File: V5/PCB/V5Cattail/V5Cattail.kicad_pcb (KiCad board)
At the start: 2 copper layers, 11 x 31.1 mm, 10 parts, among them U1 ST-0277D00-052-142, U2 SRV05-4_C558418, U3 BMI270

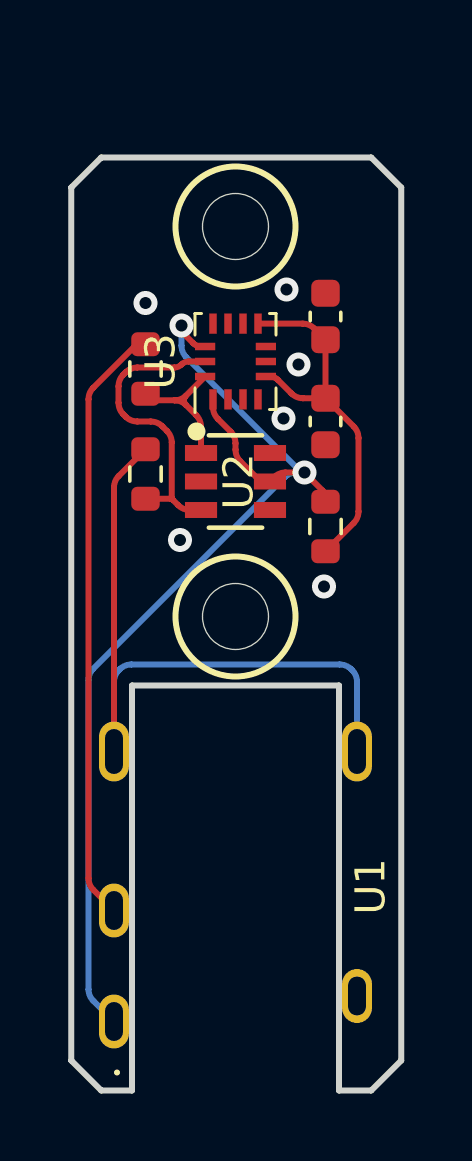
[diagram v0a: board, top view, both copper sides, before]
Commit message: Overdue backup
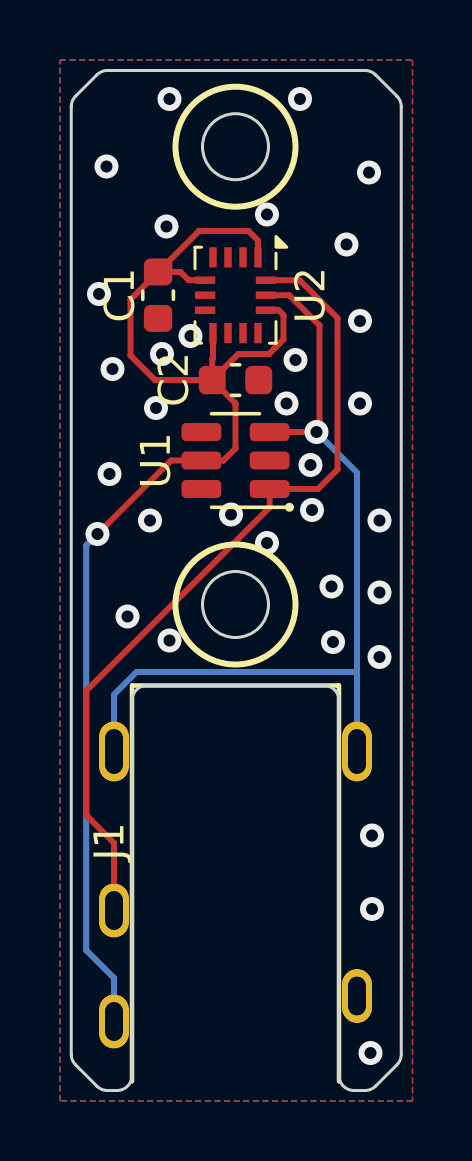
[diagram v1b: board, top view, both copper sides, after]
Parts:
- removed ? (x2): , 
- removed R1, R2, R3: 1k, Resistor_SMD:R_0603_1608Metric
- C1, C2: value 100n -> 100nF; footprint Capacitor_SMD:C_0603_1608Metric -> LilypadVR:C_0603_1608Metric
- J1: renamed from U1; value ST-0277D00-052-142 -> TRRS; footprint AUDIO-TH_ST-0277D00-052-142:AUDIO-TH_ST-0277D00-052-142 -> LilypadVR:AUDIO-TH_ST-0277D00-052-142
- U1: renamed from U2; footprint SOT-23-6_L2.9-W1.6-P0.95-LS2.8-BL:SOT-23-6_L2.9-W1.6-P0.95-LS2.8-BL -> LilypadVR:SOT-23-6
- moved C1 6.99 mm to (144.4, 86.3), turned to 90 degrees
- moved C2 3.67 mm to (147.0, 89.1), turned to 0 degrees
- moved U2 2.21 mm to (147.0, 86.3), turned to -90 degrees
- moved U1 0.70 mm to (147.0, 91.8), turned to 180 degrees
- renumbered U3 to U2
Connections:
- C1 pad 1: Net-(U3-VDD) -> GND
- C1 pad 2: GND -> +3V3
- C2 pad 1: Net-(U3-VDD) -> +3V3
- J1 pad 3: Net-(R1-Pad2) -> SDA
- J1 pad 4: Net-(R2-Pad2) -> SCL
- J1 pad 5: Net-(R2-Pad2) -> SCL
- U1 pad 1: /SDA -> SDA
- U1 pad 3: /SCL -> SCL
- U2 pad 13: /SCL -> SCL
- U2 pad 14: /SDA -> SDA
- U2 pad 5: Net-(U3-VDD) -> +3V3
- U2 pad 8: Net-(U3-VDD) -> +3V3
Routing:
- net SCL: track 0.00 -> 28.9 mm, vias 0 -> 1
- net SDA: track 0.00 -> 27.5 mm
- net Net-(R2-Pad2): track 23.9 -> 0.00 mm
- net Net-(R1-Pad2): track 20.1 -> 0.00 mm
- net Net-(U3-VDD): track 12.6 -> 0.00 mm
- net /SCL: track 10.2 -> 0.00 mm
- net +3V3: track 35.3 -> 43.7 mm, vias 2 -> 1
- net /SDA: track 4.89 -> 0.00 mm
- net GND: vias 6 -> 32
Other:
- board size 11 x 31.1 mm -> 11 x 34 mm
- rule pad_to_mask_clearance: 0 -> 0.038
